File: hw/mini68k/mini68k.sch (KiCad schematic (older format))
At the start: 29 parts, among them J1 Jack-DC, J2 6-bit input port, J3 8-bit output port, J4 FTDI header, SW1 SW_SPDT, SW2 SW_Push, U1 HM62256BLP-7, U2 68008D, U3 L7805, U4 28C256, U5 GAL16V8, U6 MAX708CPA+, U7 68681, U8 74LS05, X1 TCXO-14

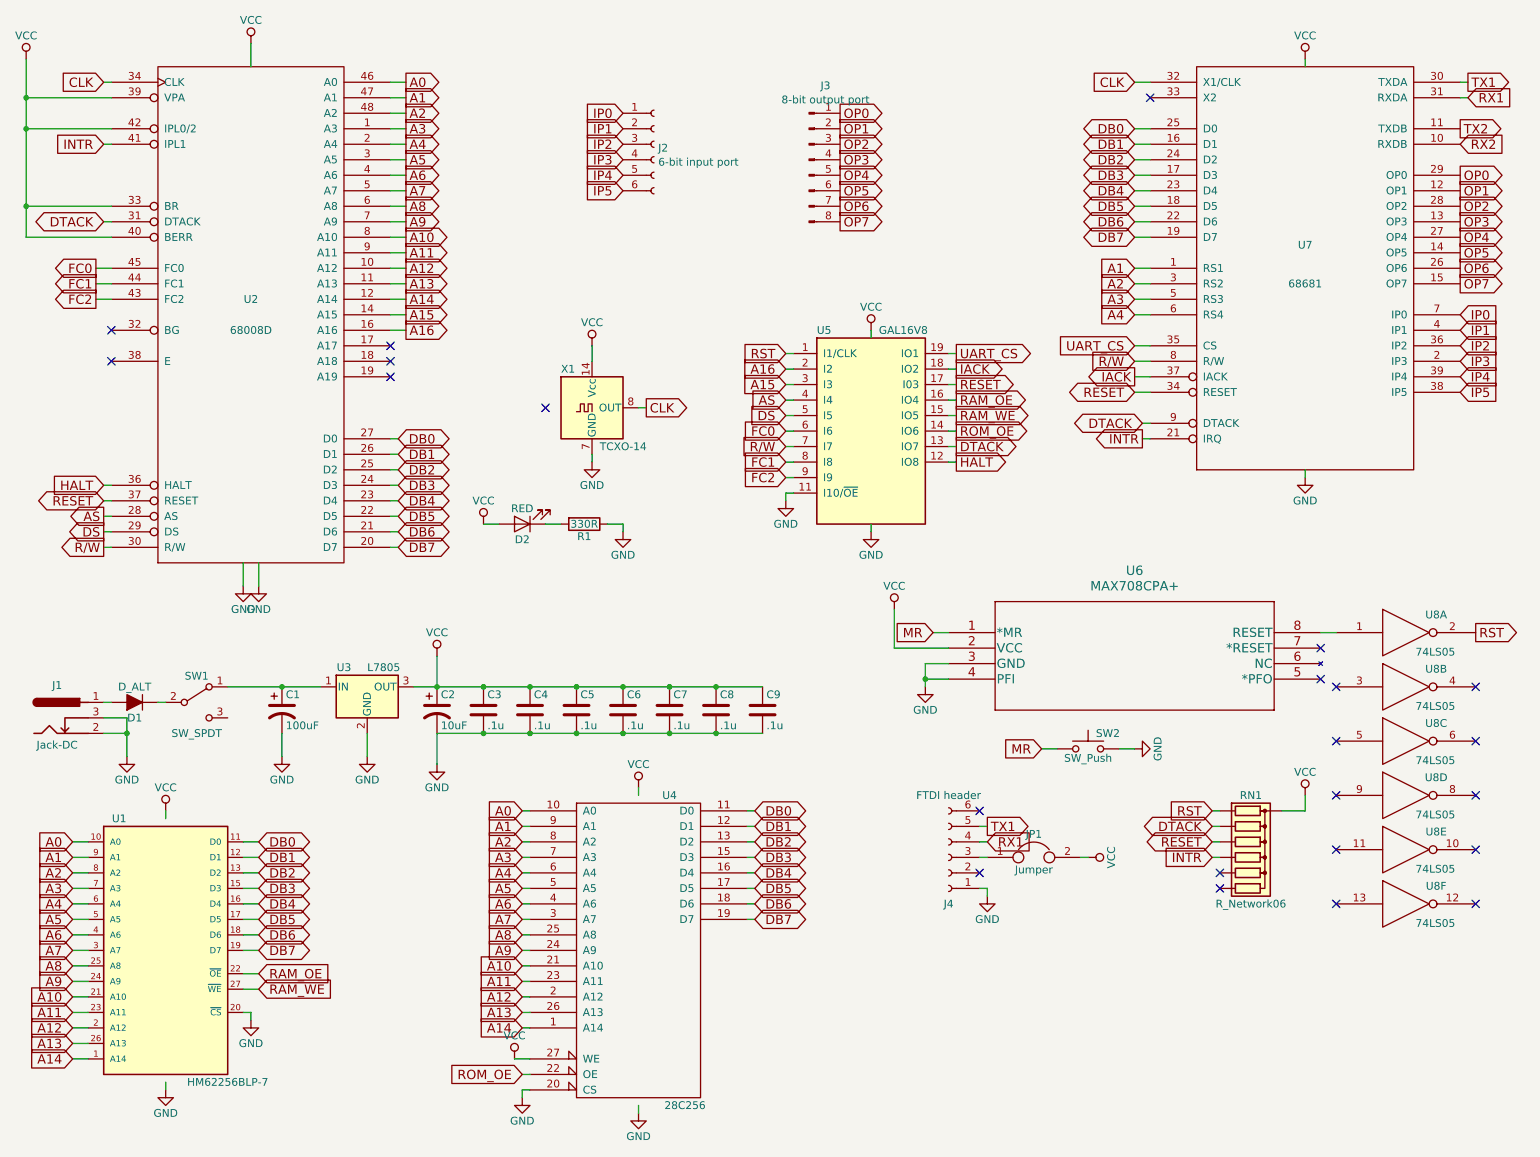
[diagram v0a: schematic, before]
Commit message: better fills
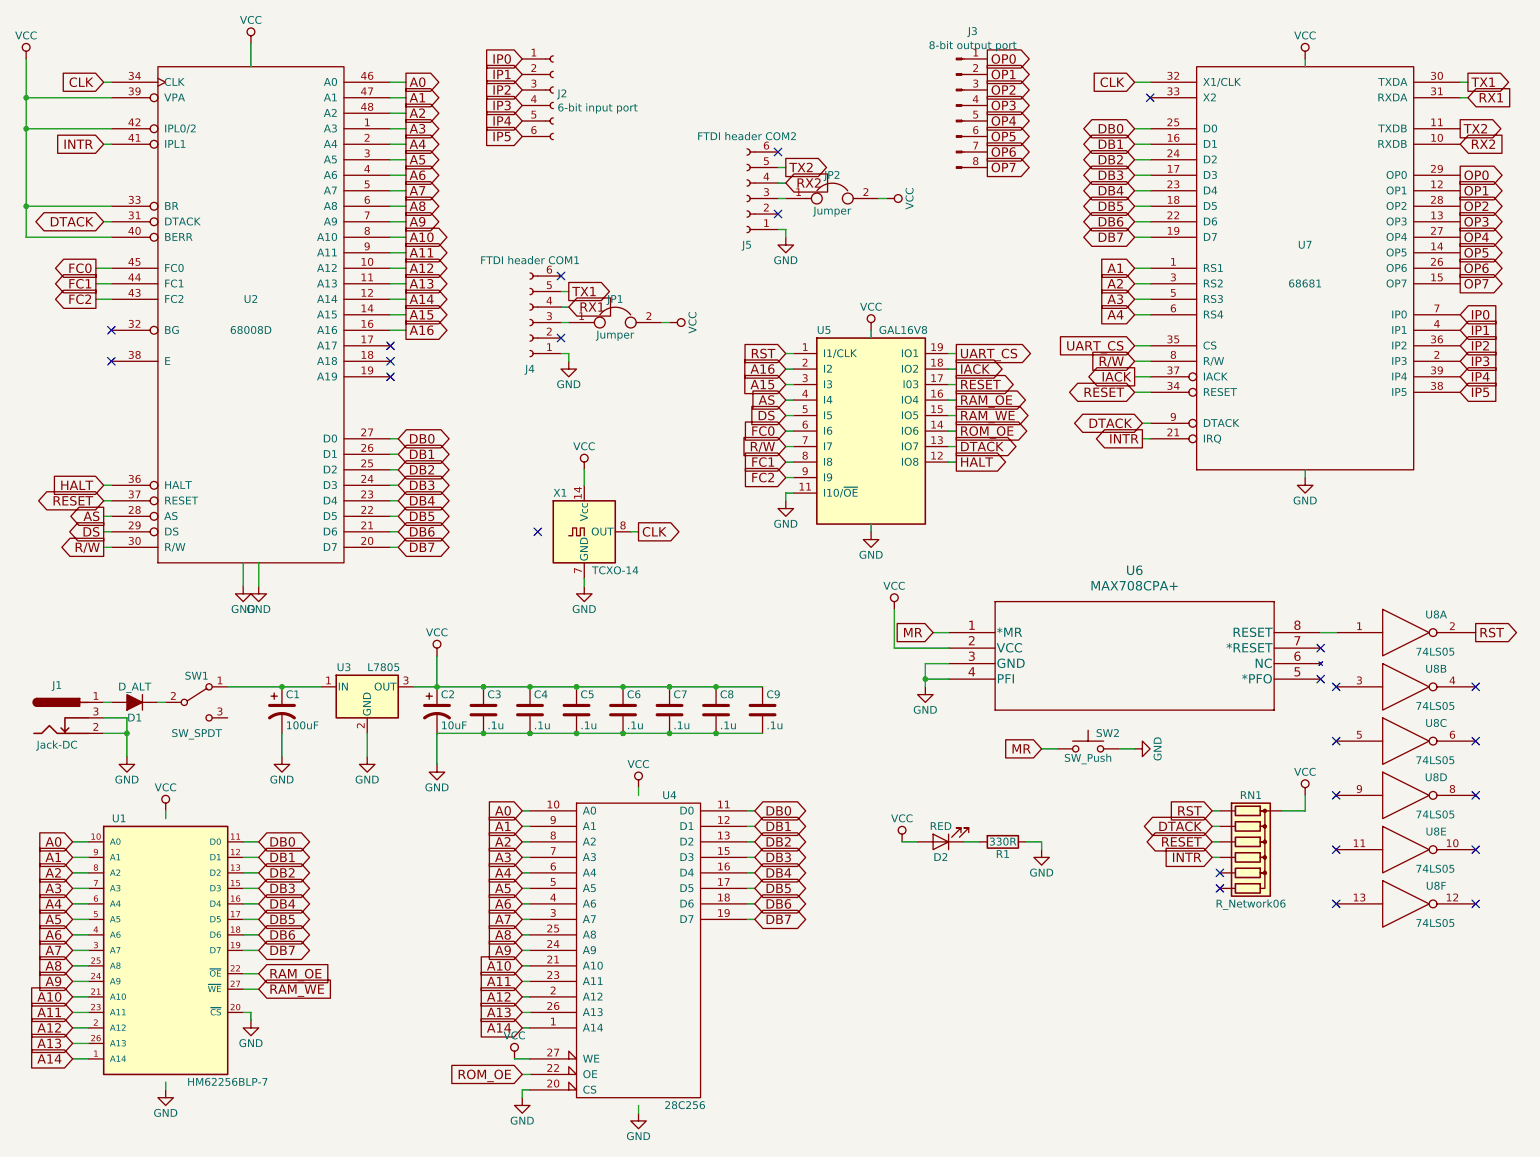
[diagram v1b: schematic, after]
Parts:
- added J5: FTDI header COM2, Connector_PinHeader_2.54mm:PinHeader_1x06_P2.54mm_Vertical, symbol mini68k-rescue:Conn_01x06_Female
- added JP2: Jumper, Connector_PinHeader_2.54mm:PinHeader_1x02_P2.54mm_Vertical, symbol Device:Jumper
- J4: value FTDI header -> FTDI header COM1
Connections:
- net GND: now also J5.1 (Pin_1)
- net RX2: now also J5.4 (Pin_4)
- net TX2: now also J5.5 (Pin_5)
- net VCC: now also JP2.2
- new net: J5.3 (Pin_3), JP2.1
- no-connect marks 23 -> 25
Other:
- moved on the sheet: D2, J2, J3, J4, JP1, R1, X1
